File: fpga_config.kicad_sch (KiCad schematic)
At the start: 17 parts, among them J2 Molex 0878321420, U2 XC7A50T-FGG484

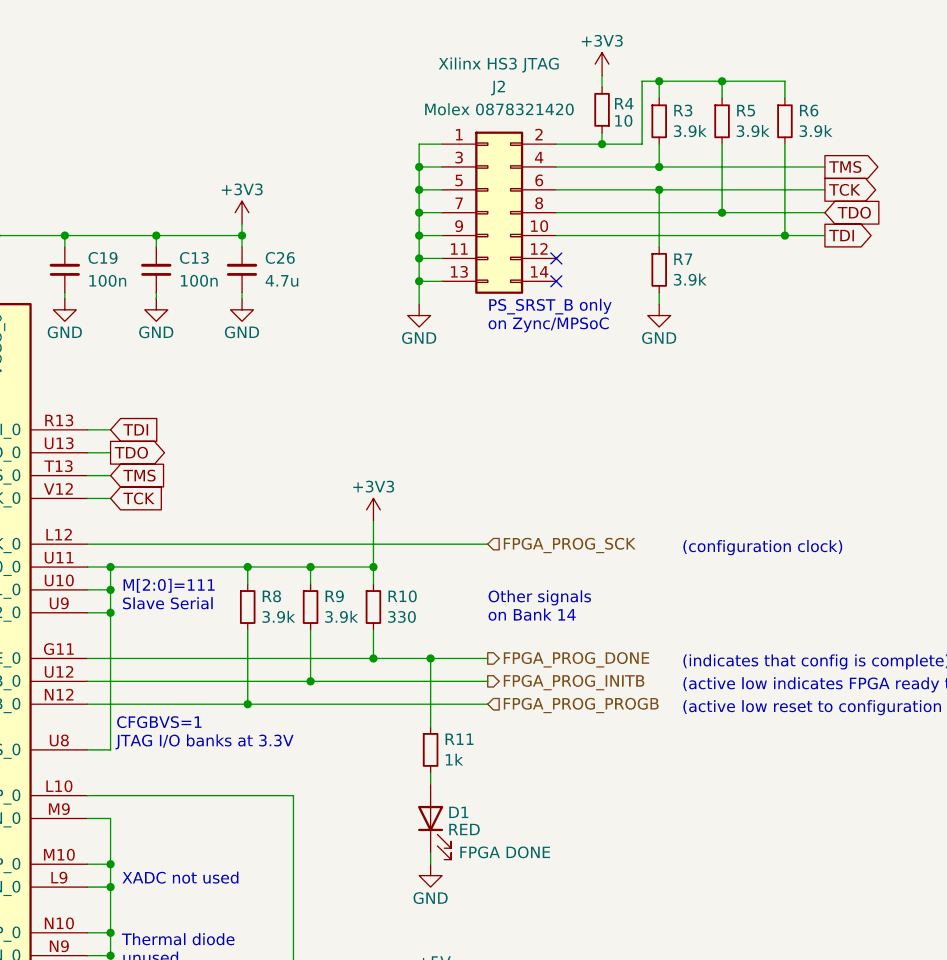
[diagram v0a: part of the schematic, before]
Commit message: Started routing. More to go
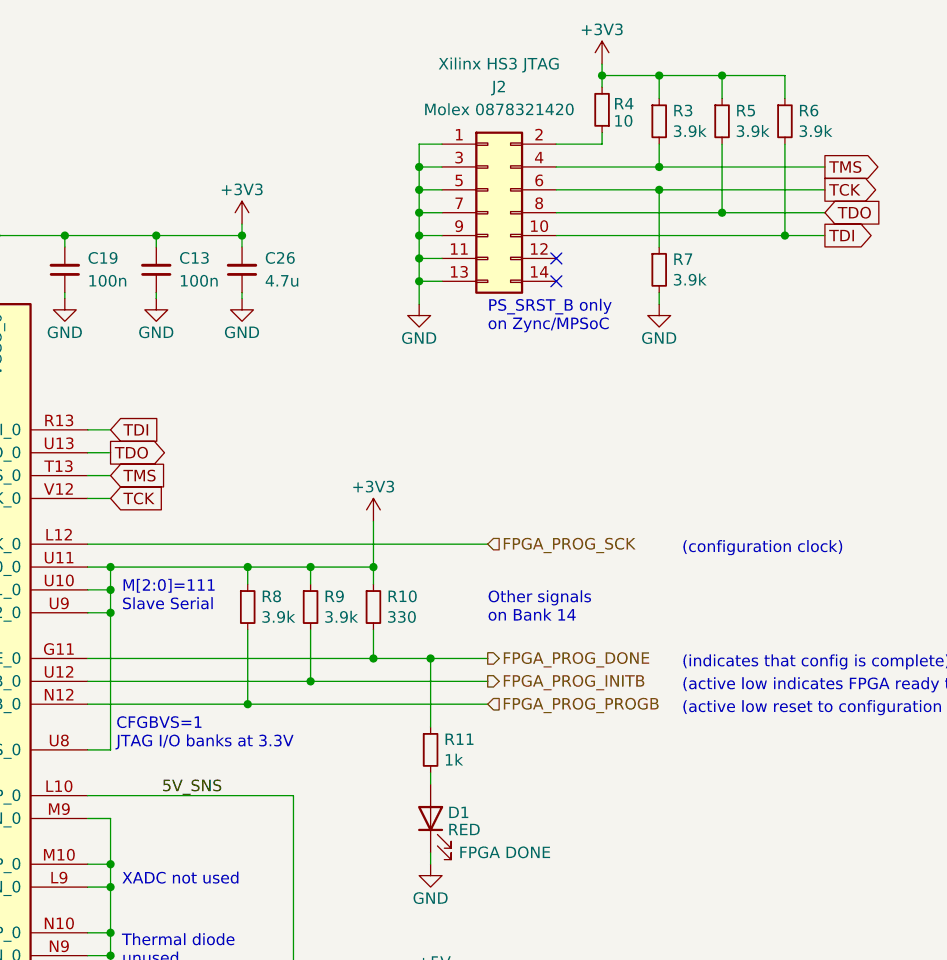
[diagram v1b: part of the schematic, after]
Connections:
- net +3V3: now also R3.1, R5.1, R6.1
- net 5V_SNS: now reaches R14.1, R15.2, U2.L10 (VP_0)
- new net: J2.2 (Pin_2), R4.1
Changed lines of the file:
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@@
   (junction (at 121.285 85.09) (diameter 0) (color 0 0 0 0)
   )
-  (junction (at 167.005 31.115) (diameter 0) (color 0 0 0 0)
+  (junction (at 167.005 30.48) (diameter 0) (color 0 0 0 0)
   )
   (junction (at 133.35 45.72) (diameter 0) (color 0 0 0 0)
@@
   (junction (at 173.99 48.26) (diameter 0) (color 0 0 0 0)
   )
-  (junction (at 160.02 31.115) (diameter 0) (color 0 0 0 0)
+  (junction (at 160.02 30.48) (diameter 0) (color 0 0 0 0)
   )
   (junction (at 114.3 85.09) (diameter 0) (color 0 0 0 0)
   )
-  (junction (at 153.67 38.1) (diameter 0) (color 0 0 0 0)
-  )
   (junction (at 133.35 53.34) (diameter 0) (color 0 0 0 0)
   )
@@
   )
   (junction (at 86.36 48.26) (diameter 0) (color 0 0 0 0)
+  )
+  (junction (at 153.67 30.48) (diameter 0) (color 0 0 0 0)
   )
   (junction (at 133.35 40.64) (diameter 0) (color 0 0 0 0)
@@
     (stroke (width 0) (type default))
   )
+  (wire (pts (xy 153.67 30.48) (xy 153.67 31.75))
+    (stroke (width 0) (type default))
+  )
   (wire (pts (xy 133.35 48.26) (xy 133.35 45.72))
     (stroke (width 0) (type default))
@@
     (stroke (width 0) (type default))
   )
-  (wire (pts (xy 167.005 31.115) (xy 173.99 31.115))
+  (wire (pts (xy 167.005 30.48) (xy 173.99 30.48))
     (stroke (width 0) (type default))
   )
@@
     (stroke (width 0) (type default))
   )
-  (wire (pts (xy 167.005 31.115) (xy 167.005 33.02))
+  (wire (pts (xy 167.005 30.48) (xy 167.005 33.02))
     (stroke (width 0) (type default))
   )
@@
     (stroke (width 0) (type default))
   )
-  (wire (pts (xy 153.67 30.48) (xy 153.67 31.75))
+  (wire (pts (xy 153.67 29.21) (xy 153.67 30.48))
     (stroke (width 0) (type default))
   )
@@
     (stroke (width 0) (type default))
   )
-  (wire (pts (xy 173.99 31.115) (xy 173.99 33.02))
+  (wire (pts (xy 173.99 30.48) (xy 173.99 33.02))
     (stroke (width 0) (type default))
   )
@@
     (stroke (width 0) (type default))
   )
-  (wire (pts (xy 160.02 31.115) (xy 167.005 31.115))
+  (wire (pts (xy 160.02 30.48) (xy 167.005 30.48))
     (stroke (width 0) (type default))
   )
@@
     (stroke (width 0) (type default))
   )
-  (wire (pts (xy 160.02 31.115) (xy 160.02 33.02))
+  (wire (pts (xy 160.02 30.48) (xy 160.02 33.02))
     (stroke (width 0) (type default))
   )
@@
     (stroke (width 0) (type default))
   )
-  (wire (pts (xy 153.67 38.1) (xy 158.115 38.1))
-    (stroke (width 0) (type default))
-  )
   (wire (pts (xy 134.62 147.32) (xy 134.62 148.59))
     (stroke (width 0) (type default))
@@
     (stroke (width 0) (type default))
   )
-  (wire (pts (xy 158.115 31.115) (xy 160.02 31.115))
+  (wire (pts (xy 153.67 30.48) (xy 160.02 30.48))
     (stroke (width 0) (type default))
   )
@@
   )
   (wire (pts (xy 96.52 74.93) (xy 99.06 74.93))
-    (stroke (width 0) (type default))
-  )
-  (wire (pts (xy 158.115 38.1) (xy 158.115 31.115))
     (stroke (width 0) (type default))
   )
@@
     (effects (font (size 1.27 1.27)) (justify left bottom))
   )
+  (label "5V_SNS" (at 104.775 110.49 0) (fields_autoplaced)
+    (effects (font (size 1.27 1.27)) (justify left bottom))
+  )
   (global_label "TMS" (shape output) (at 178.435 40.64 0) (fields_autoplaced)
     (effects (font (size 1.27 1.27)) (justify left))
@@
     )
   )
-  (symbol (lib_id "power:+3V3") (at 153.67 30.48 0) (unit 1)
+  (symbol (lib_id "power:+3V3") (at 153.67 29.21 0) (unit 1)
     (in_bom yes) (on_board yes) (dnp no)
-    (property "Reference" "#PWR020" (at 153.67 34.29 0)
-      (effects (font (size 1.27 1.27)) hide)
-    )
-    (property "Value" "+3V3" (at 153.67 26.67 0)
+    (property "Reference" "#PWR020" (at 153.67 33.02 0)
+      (effects (font (size 1.27 1.27)) hide)
+    )
+    (property "Value" "+3V3" (at 153.67 25.4 0)
       (effects (font (size 1.27 1.27)))
     )
-    (property "Footprint" "" (at 153.67 30.48 0)
-      (effects (font (size 1.27 1.27)) hide)
-    )
-    (property "Datasheet" "" (at 153.67 30.48 0)
-      (effects (font (size 1.27 1.27)) hide)
-    )
+    (property "Footprint" "" (at 153.67 29.21 0)
+      (effects (font (size 1.27 1.27)) hide)
+    )
+    (property "Datasheet" "" (at 153.67 29.21 0)
+      (effects (font (size 1.27 1.27)) hide)
+    )
